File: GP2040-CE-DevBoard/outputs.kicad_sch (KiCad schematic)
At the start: 10 parts, among them J3 Debug, J4 RGB LED

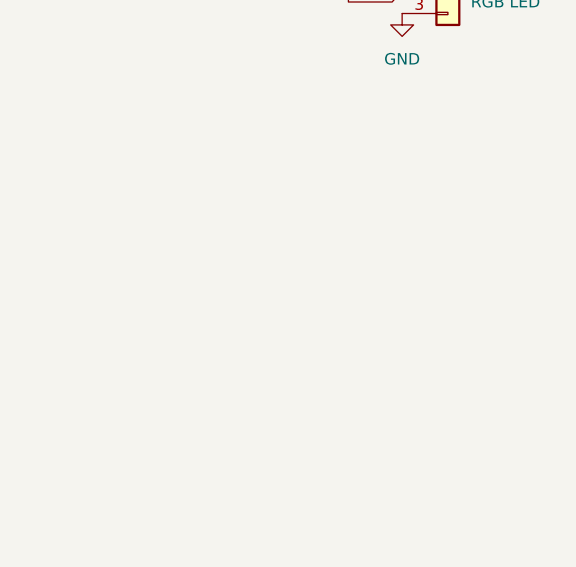
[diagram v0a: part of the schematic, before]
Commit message: Updating schema and PCB design
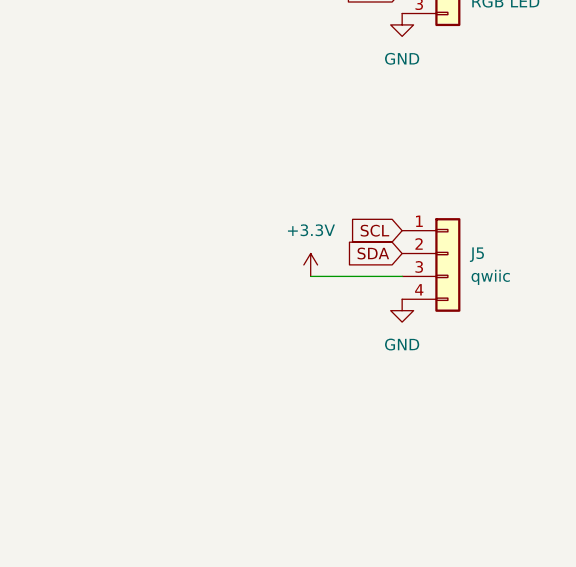
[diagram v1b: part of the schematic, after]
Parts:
- added J5: qwiic, Connector_JST:JST_SH_BM04B-SRSS-TB_1x04-1MP_P1.00mm_Vertical, symbol Connector_Generic:Conn_01x04
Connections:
- net GND: now also J5.4 (Pin_4)
- new net +3V3: J5.3 (Pin_3)
- new net SCL: J5.1 (Pin_1)
- new net SDA: J5.2 (Pin_2)
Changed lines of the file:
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@@
+    (stroke (width 0) (type default) (color 0 0 0 0))
+  )
+  (wire (pts (xy 97.79 60.96) (xy 107.95 60.96))
     (stroke (width 0) (type default) (color 0 0 0 0))
   )
@@
     )
   )
+  (global_label "SDA" (shape input) (at 107.95 58.42 180) (fields_autoplaced)
+    (effects (font (size 1.27 1.27)) (justify right))
+    (property "Intersheet References" "${INTERSHEET_REFS}" (id 0) (at 101.9688 58.3406 0)
+      (effects (font (size 1.27 1.27)) (justify right) hide)
+    )
+  )
   (global_label "PLED1" (shape input) (at 44.45 69.85 270) (fields_autoplaced)
     (effects (font (size 1.27 1.27)) (justify right))
     (property "Intersheet References" "${INTERSHEET_REFS}" (id 0) (at 44.3706 78.1898 90)
+      (effects (font (size 1.27 1.27)) (justify right) hide)
+    )
+  )
+  (global_label "SCL" (shape input) (at 107.95 55.88 180) (fields_autoplaced)
+    (effects (font (size 1.27 1.27)) (justify right))
+    (property "Intersheet References" "${INTERSHEET_REFS}" (id 0) (at 102.0293 55.8006 0)
       (effects (font (size 1.27 1.27)) (justify right) hide)
     )
@@
     (pin "3")
   )
+  (symbol (lib_id "power:GND") (at 107.95 63.5 0) (unit 1)
+    (in_bom yes) (on_board yes) (fields_autoplaced)
+    (property "Reference" "#PWR070" (id 0) (at 107.95 69.85 0)
+      (effects (font (size 1.27 1.27)) hide)
+    )
+    (property "Value" "GND" (id 1) (at 107.95 68.58 0))
+    (property "Footprint" "" (id 2) (at 107.95 63.5 0)
+      (effects (font (size 1.27 1.27)) hide)
+    )
+    (property "Datasheet" "" (id 3) (at 107.95 63.5 0)
+      (effects (font (size 1.27 1.27)) hide)
+    )
+    (pin "1")
+  )
   (symbol (lib_id "power:GND") (at 33.02 62.23 0) (unit 1)
     (in_bom yes) (on_board yes) (fields_autoplaced)
@@
   (symbol (lib_id "power:GND") (at 107.95 31.75 0) (unit 1)
     (in_bom yes) (on_board yes) (fields_autoplaced)
-    (property "Reference" "#PWR068" (id 0) (at 107.95 38.1 0)
+    (property "Reference" "#PWR069" (id 0) (at 107.95 38.1 0)
       (effects (font (size 1.27 1.27)) hide)
     )
@@
   (symbol (lib_id "power:VBUS") (at 107.95 26.67 0) (unit 1)
     (in_bom yes) (on_board yes) (fields_autoplaced)
-    (property "Reference" "#PWR067" (id 0) (at 107.95 30.48 0)
+    (property "Reference" "#PWR068" (id 0) (at 107.95 30.48 0)
       (effects (font (size 1.27 1.27)) hide)
     )
@@
     (pin "2")
   )
+  (symbol (lib_id "Connector_Generic:Conn_01x04") (at 113.03 58.42 0) (unit 1)
+    (in_bom yes) (on_board yes) (fields_autoplaced)
+    (property "Reference" "J5" (id 0) (at 115.57 58.4199 0)
+      (effects (font (size 1.27 1.27)) (justify left))
+    )
+    (property "Value" "qwiic" (id 1) (at 115.57 60.9599 0)
+      (effects (font (size 1.27 1.27)) (justify left))
+    )
+    (property "Footprint" "Connector_JST:JST_SH_BM04B-SRSS-TB_1x04-1MP_P1.00mm_Vertical" (id 2) (at 113.03 58.42 0)
+      (effects (font (size 1.27 1.27)) hide)
+    )
+    (property "Datasheet" "~" (id 3) (at 113.03 58.42 0)
+      (effects (font (size 1.27 1.27)) hide)
+    )
+    (pin "1")
+    (pin "2")
+    (pin "3")
+    (pin "4")
+  )
   (symbol (lib_id "Device:R") (at 44.45 132.08 0) (unit 1)
     (in_bom yes) (on_board yes) (fields_autoplaced)
@@
       (effects (font (size 1.27 1.27)) hide)
     )
+    (pin "1")
+  )
+  (symbol (lib_id "power:+3.3V") (at 97.79 60.96 0) (unit 1)
+    (in_bom yes) (on_board yes) (fields_autoplaced)
+    (property "Reference" "#PWR067" (id 0) (at 97.79 64.77 0)
+      (effects (font (size 1.27 1.27)) hide)
+    )
+    (property "Value" "+3.3V" (id 1) (at 97.79 55.88 0))
+    (property "Footprint" "" (id 2) (at 97.79 60.96 0)
+      (effects (font (size 1.27 1.27)) hide)
+    )
+    (property "Datasheet" "" (id 3) (at 97.79 60.96 0)
+      (effects (font (size 1.27 1.27)) hide)
+    )
